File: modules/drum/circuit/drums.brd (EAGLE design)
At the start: 178.7 x 113 mm, 122 parts, among them IC1 LM324N, IC2 LM324N, Q1 2N3904, Q2 2N3904, Q3 2N3904

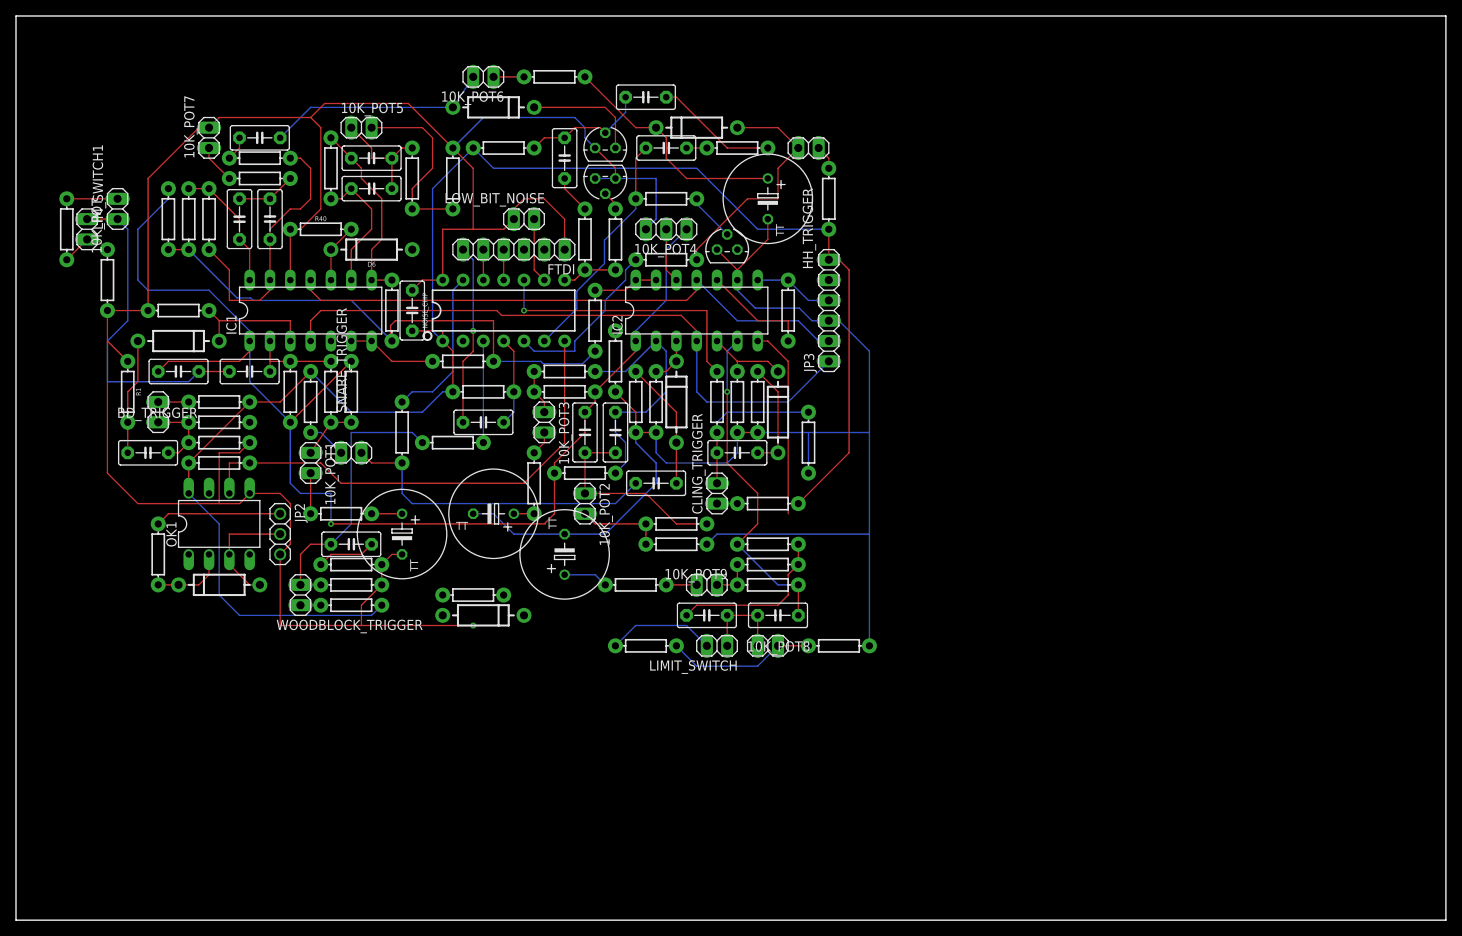
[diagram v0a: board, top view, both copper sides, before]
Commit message: drum machine
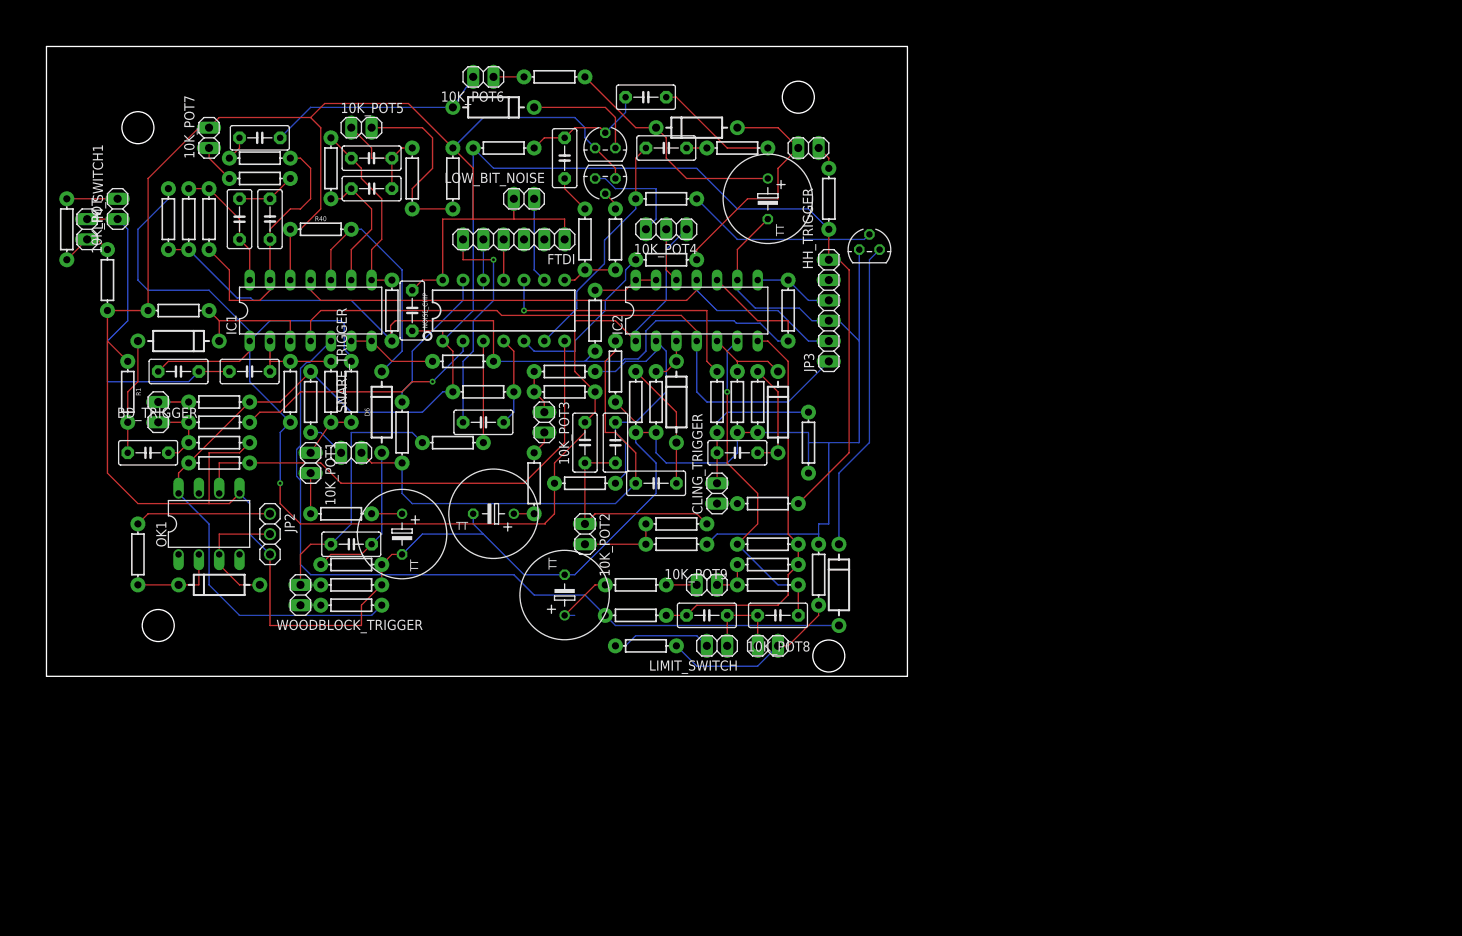
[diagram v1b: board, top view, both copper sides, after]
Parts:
- moved D8 44.6 mm to (102.9, 8.89), turned to 90 degrees
- moved R59 20.5 mm to (77.5, 5.08)
- moved D6 20.4 mm to (45.7, 30.5), turned to 90 degrees
- moved Q3 17.8 mm to (106.7, 50.8)
- moved R50 9.25 mm to (100.3, 10.2), turned to 270 degrees
- moved C23 5.08 mm to (68.6, 7.62)
- moved 10K_POT2 3.81 mm to (71.1, 15.2)
- moved 1M2 2.54 mm to (15.2, 12.7)
- moved LOW_BIT_NOISE 2.54 mm to (63.5, 57.1)
- moved FTDI 1.27 mm to (62.2, 52.1)
- moved JP2 1.27 mm to (31.8, 15.2)
- moved C6 1.27 mm to (74.9, 26.7)
- moved C7 1.27 mm to (71.1, 26.7)
- moved OK1 1.27 mm to (24.1, 16.5)
- moved R13 1.27 mm to (71.1, 21.6)
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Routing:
- net N$53: track 0.00 -> 100.6 mm
- net N$52: track 0.00 -> 38.9 mm
- net BD_TRIGGER: track 0.00 -> 31.6 mm, vias 0 -> 1
- net N$34: track 79.9 -> 109.7 mm
- net N$28: track 7.40 -> 29.6 mm
- net N$25: track 40.2 -> 60.8 mm
- net BD_OUT: track 155.6 -> 174.2 mm
- net N$51: track 6.66 -> 24.6 mm
- net GND: track 444.8 -> 431.9 mm, vias 1 -> 0
- net N$49: track 7.40 -> 19.4 mm
- net BD_OUT1: track 44.5 -> 51.4 mm
- net RESET: track 22.6 -> 28.2 mm
- net N$13: track 18.6 -> 22.7 mm
- net RX: track 3.81 -> 6.35 mm
- net N$60: track 8.15 -> 10.7 mm
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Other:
- board size 178.7 x 113 mm -> 107.6 x 78.7 mm

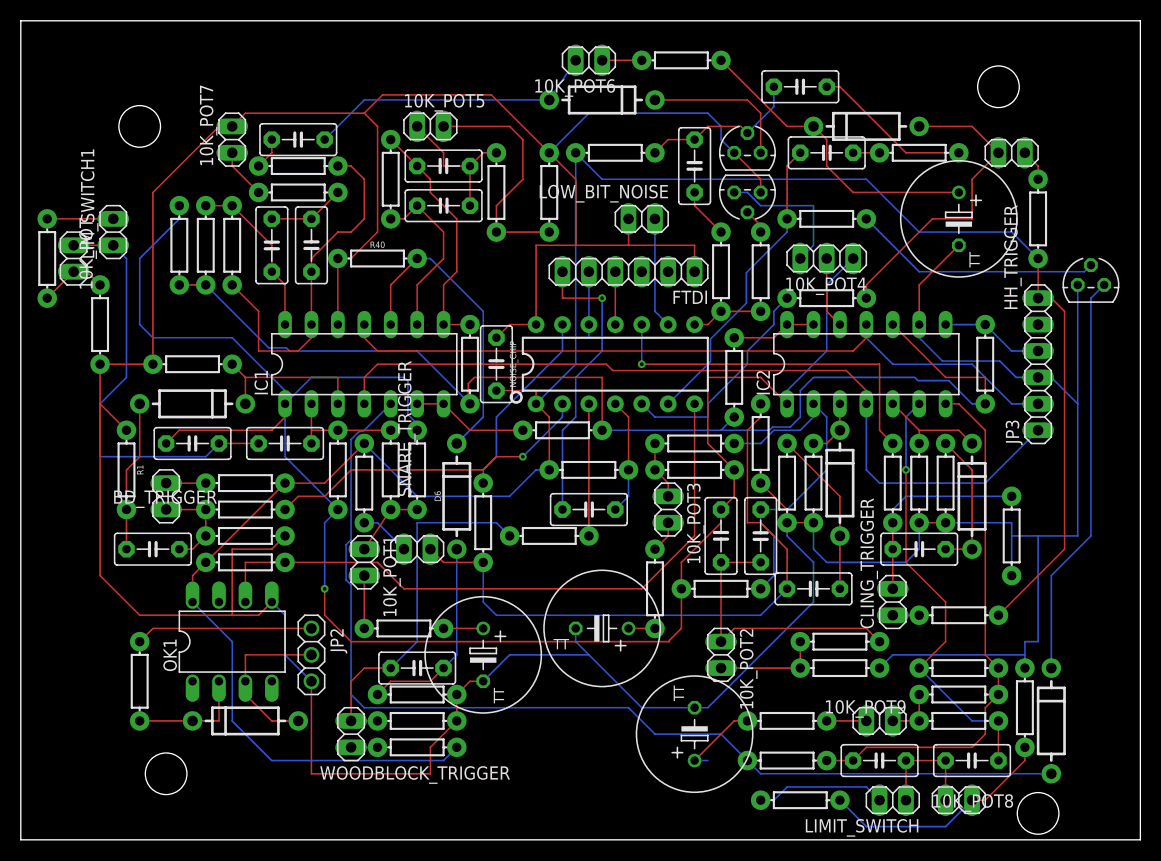
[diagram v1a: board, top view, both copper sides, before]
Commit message: long overdue commit
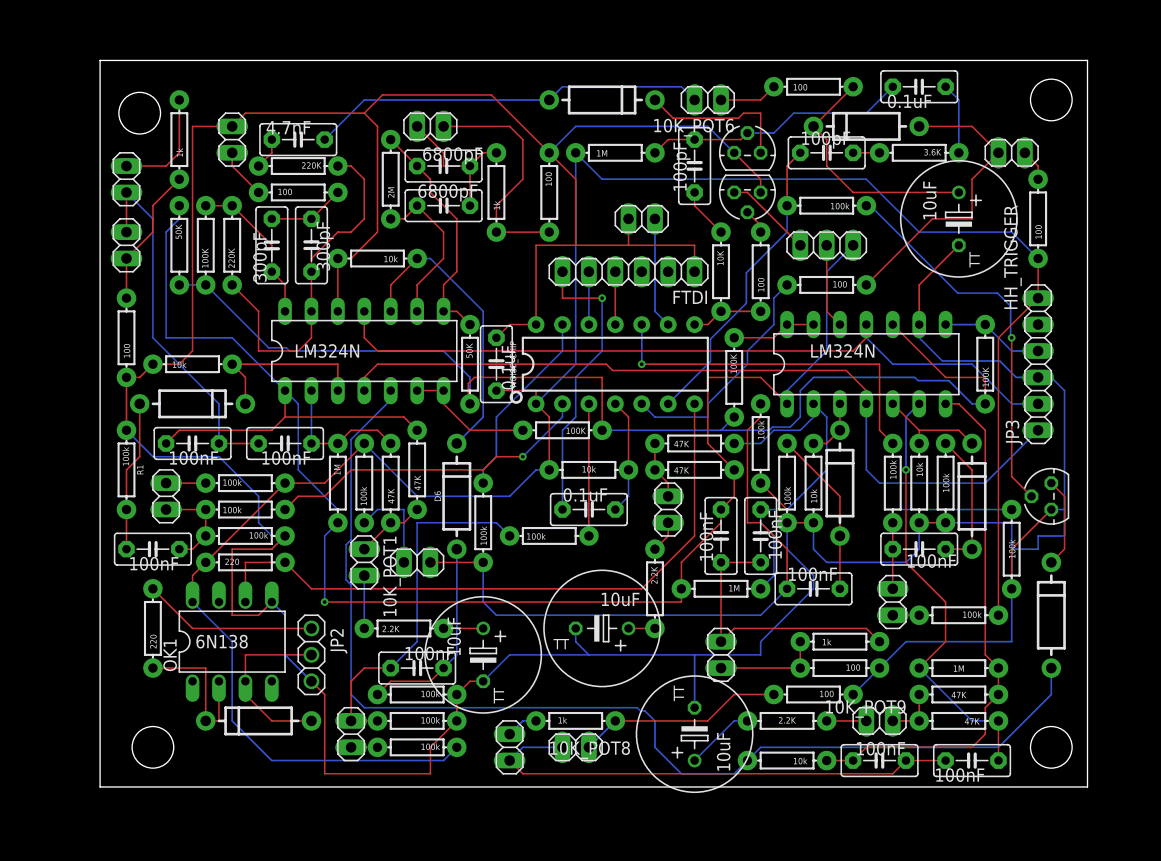
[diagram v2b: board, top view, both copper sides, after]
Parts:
- moved 10K_POT8 37.2 mm to (57.1, 6.35)
- moved LIMIT_SWITCH 37.2 mm to (50.8, 6.35), turned to 90 degrees
- moved R49 22.9 mm to (57.1, 8.89)
- moved Q3 20.7 mm to (102.9, 30.5), turned to 90 degrees
- moved R50 20.4 mm to (80.0, 11.4), turned to 180 degrees
- moved R6 17.1 mm to (19.1, 64.8)
- moved R26 13.0 mm to (80.0, 69.8)
- moved 10K_POT6 12.0 mm to (69.8, 68.6)
- moved C12 11.4 mm to (90.2, 69.8)
- moved D8 10.2 mm to (102.9, 19.1)
- moved 1M2 5.24 mm to (16.5, 17.8)
- moved 10K_POT 5.24 mm to (14.0, 54.6)
- moved LIM_SWITCH1 5.24 mm to (14.0, 61.0)
- moved R7 2.84 mm to (14.0, 45.7)
- moved D2 1.27 mm to (26.7, 8.89)
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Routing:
- net N$1: track 11.4 -> 48.6 mm
- net N$52: track 38.9 -> 8.67 mm
- net GND: track 431.9 -> 408.9 mm
- net N$51: track 24.6 -> 37.0 mm, vias 0 -> 1
- net N$59: track 13.8 -> 3.07 mm
- net BD_OUT: track 174.2 -> 163.5 mm
- net N$36: track 27.7 -> 38.2 mm
- net N$40: track 16.6 -> 25.5 mm
- net N$39: track 15.3 -> 6.88 mm
- net N$53: track 100.6 -> 108.8 mm
- net N$9: track 6.66 -> 13.5 mm
- net N$33: track 29.6 -> 23.5 mm
- net N$6: track 41.5 -> 35.4 mm
- net N$23: track 13.8 -> 8.45 mm
- net N$27: track 4.86 -> 9.42 mm
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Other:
- board size 107.6 x 78.7 mm -> 94.9 x 69.8 mm
